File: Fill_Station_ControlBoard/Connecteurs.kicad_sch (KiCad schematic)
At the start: 44 parts, among them J1 RJ45_Wuerth_7499010211A, U1 LAN8742A, Y3 ASV-25.000MHz

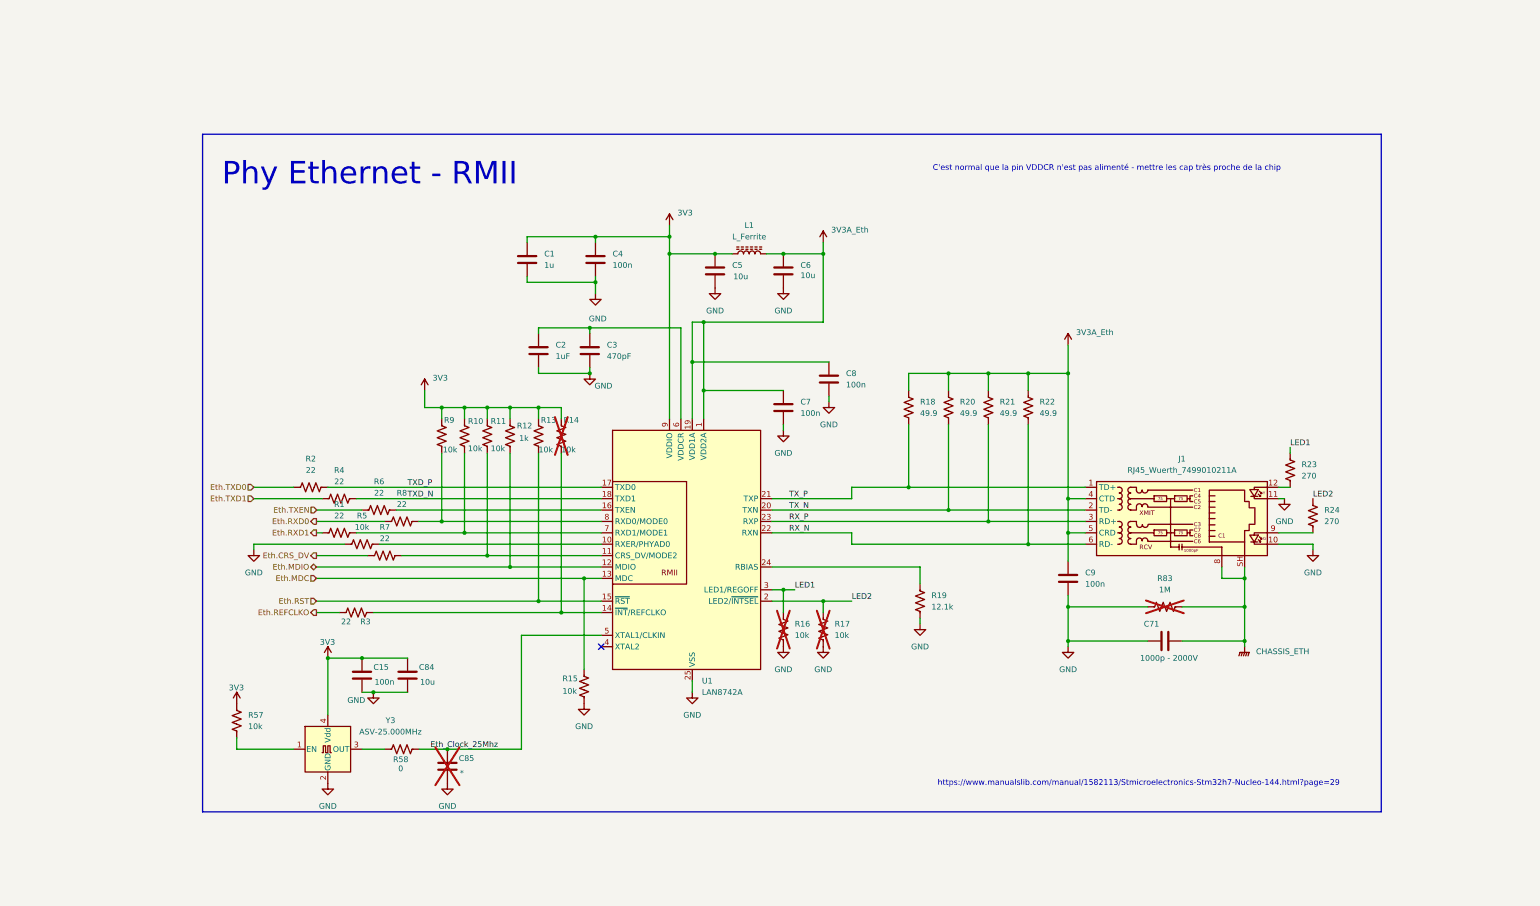
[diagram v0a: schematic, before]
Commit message: Travail Layout
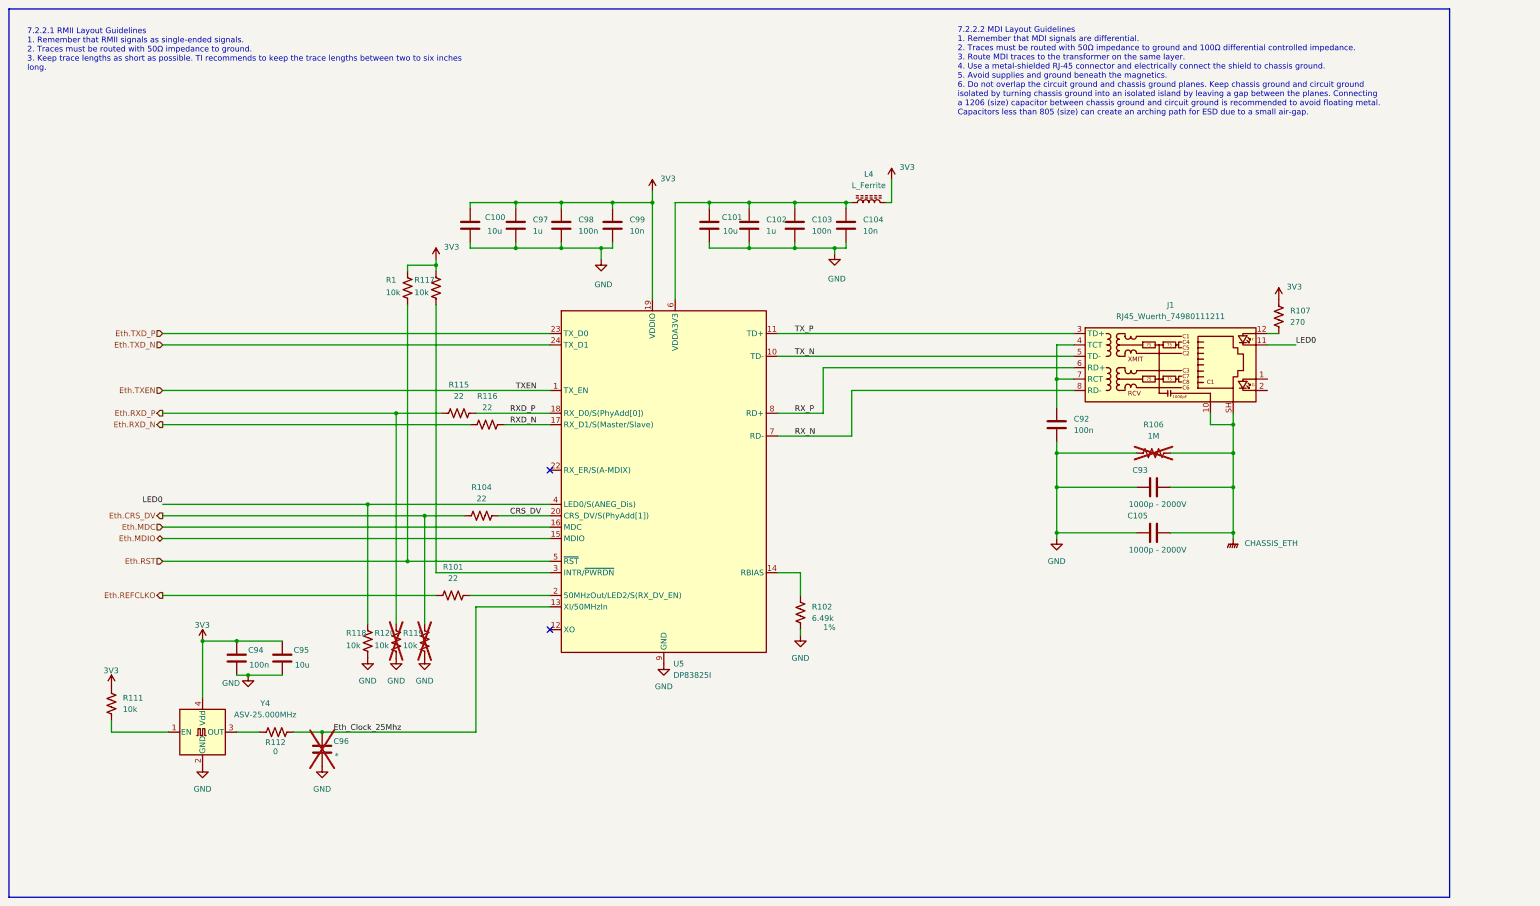
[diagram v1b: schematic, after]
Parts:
- removed C1: 1u, Capacitor_SMD:C_0603_1608Metric, symbol Device:C
- removed C15, C9: 100n, Capacitor_SMD:C_0402_1005Metric, symbol Device:C
- removed C2: 1uF, Capacitor_SMD:C_0603_1608Metric, symbol Device:C
- removed C3: 470pF, Capacitor_SMD:C_0603_1608Metric, symbol Device:C
- removed C4: 100n, Capacitor_SMD:C_0603_1608Metric, symbol Device:C
- removed C5, C6: 10u, Capacitor_SMD:C_0603_1608Metric, symbol Device:C
- removed C7, C8: 100n, Resistor_SMD:R_0402_1005Metric, symbol Device:C
- removed C71: 1000p - 2000V, Capacitor_SMD:C_1210_3225Metric, symbol Device:C
- removed C84: 10u, Capacitor_SMD:C_0402_1005Metric, symbol Device:C
- removed C85: *, Capacitor_SMD:C_0402_1005Metric, symbol Device:C
- removed J1: RJ45_Wuerth_7499010211A, Connector_RJ:RJ45_Wuerth_7499010211A_Horizontal, symbol Connector:RJ45_Wuerth_7499010211A
- removed L1: L_Ferrite, Capacitor_SMD:C_0402_1005Metric, symbol Device:L_Ferrite
- removed R10, R11, R13, R14, R15, R16, R17, R5, R9: 10k, Resistor_SMD:R_0603_1608Metric_Pad0.98x0.95mm_HandSolder, symbol Device:R_US
- removed R12: 1k, Resistor_SMD:R_0603_1608Metric_Pad0.98x0.95mm_HandSolder, symbol Device:R_US
- removed R18, R20, R21, R22: 49.9, Resistor_SMD:R_0603_1608Metric_Pad0.98x0.95mm_HandSolder, symbol Device:R_US
- removed R19: 12.1k, Resistor_SMD:R_0402_1005Metric, symbol Device:R_US
- removed R2, R3, R4, R6, R7, R8: 22, Resistor_SMD:R_0402_1005Metric, symbol Device:R_US
- removed R23, R24: 270, Resistor_SMD:R_0603_1608Metric_Pad0.98x0.95mm_HandSolder, symbol Device:R_US
- removed R57: 10k, Capacitor_SMD:C_0402_1005Metric, symbol Device:R_US
- removed R58: 0, Capacitor_SMD:C_0402_1005Metric, symbol Device:R_US
- removed R83: 1M, Resistor_SMD:R_0603_1608Metric_Pad0.98x0.95mm_HandSolder, symbol Device:R_US
- removed U1: LAN8742A, Package_DFN_QFN:VQFN-24-1EP_4x4mm_P0.5mm_EP2.5x2.5mm_ThermalVias, symbol Interface_Ethernet:LAN8742A
- removed Y3: ASV-25.000MHz, Oscillator:Oscillator_SMD_Abracon_ASV-4Pin_7.0x5.1mm, symbol Oscillator:ASV-xxxMHz
- added C100, C101: 10u, Capacitor_SMD:C_0603_1608Metric, symbol Device:C
- added C102, C97: 1u, Capacitor_SMD:C_0603_1608Metric, symbol Device:C
- added C103, C92, C94, C98: 100n, Capacitor_SMD:C_0402_1005Metric, symbol Device:C
- added C104, C99: 10n, Capacitor_SMD:C_0402_1005Metric, symbol Device:C
- added C105, C93: 1000p - 2000V, Capacitor_SMD:C_1210_3225Metric, symbol Device:C
- added C95: 10u, Capacitor_SMD:C_0402_1005Metric, symbol Device:C
- added C96: *, Capacitor_SMD:C_0402_1005Metric, symbol Device:C
- added J1: RJ45_Wuerth_74980111211, Connector_RJ:RJ45_Wuerth_74980111211_Horizontal, symbol Connector:RJ45_Wuerth_74980111211
- added L4: L_Ferrite, Capacitor_SMD:C_0402_1005Metric, symbol Device:L_Ferrite
- added R101, R104, R115, R116: 22, Resistor_SMD:R_0402_1005Metric, symbol Device:R_US
- added R102: 6.49k, Resistor_SMD:R_0402_1005Metric, symbol Device:R_US
- added R106: 1M, Resistor_SMD:R_0603_1608Metric_Pad0.98x0.95mm_HandSolder, symbol Device:R_US
- added R107: 270, Resistor_SMD:R_0603_1608Metric_Pad0.98x0.95mm_HandSolder, symbol Device:R_US
- added R111: 10k, Capacitor_SMD:C_0402_1005Metric, symbol Device:R_US
- added R112: 0, Capacitor_SMD:C_0402_1005Metric, symbol Device:R_US
- added R117, R118, R119, R120: 10k, Resistor_SMD:R_0603_1608Metric_Pad0.98x0.95mm_HandSolder, symbol Device:R_US
- added U5: DP83825I, Package_DFN_QFN:Texas_RMQ0024A_WQFN-24-1EP_3x3mm_P0.4mm_EP1.9x1.9mm, symbol Interface_Ethernet:DP83825I
- added Y4: ASV-25.000MHz, Oscillator:Oscillator_SMD_Abracon_ASV-4Pin_7.0x5.1mm, symbol Oscillator:ASV-xxxMHz
- R1: value 22 -> 10k; footprint Resistor_SMD:R_0402_1005Metric -> Resistor_SMD:R_0603_1608Metric_Pad0.98x0.95mm_HandSolder
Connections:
- net Eth.RXD1 is gone; now on net 3V3: R1.1
- net 3V3: now also C100.1, C94.1, C95.1, C97.1, C98.1, C99.1, L4.2, R107.1, R111.1, R117.1, U5.19 (VDDIO), Y4.4 (Vdd)
- net CHASSIS_ETH: now also C105.2, C93.2, J1.10, J1.SH, R106.2
- net Eth.CRS_DV: now also R104.1, R119.1
- net Eth.MDC: now also U5.16 (MDC)
- net Eth.MDIO: now also U5.15 (MDIO)
- net Eth.REFCLKO: now also R101.1
- net Eth.RST: now also R1.2, U5.5 (~{RST})
- net Eth.TXEN: now also U5.1 (TX_EN)
- net Eth_Clock_25Mhz: now also C96.1, R112.2, U5.13 (XI/50MHzIn)
- net GND: now also C100.2, C101.2, C102.2, C103.2, C104.2, C105.1, C92.2, C93.1, C94.2, C95.2, C96.2, C97.2, C98.2, C99.2, R102.2, R106.1, R118.2, R119.2, R120.2, U5.21 (GND), U5.25 (GND), U5.9 (GND), Y4.2 (GND)
- net RX_N: now also J1.8 (RD-), U5.7 (RD-)
- net RX_P: now also J1.6 (RD+), U5.8 (RD+)
- net TX_N: now also J1.5 (TD-), U5.10 (TD-)
- net TX_P: now also J1.3 (TD+), U5.11 (TD+)
- new net: C101.1, C102.1, C103.1, C104.1, L4.1, U5.6 (VDDA3V3)
- new net: R111.2, Y4.1 (EN)
- new net: R112.1, Y4.3 (OUT)
- new net: J1.12, R107.2
- new net: C92.1, J1.4 (TCT), J1.7 (RCT)
- new net: R101.2, U5.2 (50MHzOut/LED2/S(RX_DV_EN))
- new net: R102.1, U5.14 (RBIAS)
- new net: R117.2, U5.3 (INTR/~{PWRDN})
- new net CRS_DV: R104.2, U5.20 (CRS_DV/S(PhyAdd[1]))
- new net Eth.RXD_N: R116.1
- new net Eth.RXD_P: R115.1, R120.1
- new net Eth.TXD_N: U5.24 (TX_D1)
- new net Eth.TXD_P: U5.23 (TX_D0)
- new net LED0: J1.11, R118.1, U5.4 (LED0/S(ANEG_Dis))
- new net RXD_N: R116.2, U5.17 (RX_D1/S(Master/Slave))
- new net RXD_P: R115.2, U5.18 (RX_D0/S(PhyAdd[0]))
- no-connect marks 1 -> 2
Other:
- note added: "7.2.2.1 RMII Layout Guidelines 1. Remember that RMII signals as single-ended signals. 2. Traces must be routed with 50Ω impedance to ground. 3. Keep trace lengths as short as possible. TI recommends to keep the trace lengths between two to six inches long."
- note added: "7.2.2.2 MDI Layout Guidelines 1. Remember that MDI signals are differential. 2. Traces must be routed with 50Ω impedance to ground and 100Ω differential controlled impedance. 3. Route MDI traces to the transformer on the same layer. 4. Use a metal-shielded RJ-45 connector and electrically connect the shield to chassis ground. 5. Avoid supplies and ground beneath the magnetics. 6. Do not overlap t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"
- note removed: "C'est normal que la pin VDDCR n'est pas alimenté - mettre les cap très proche de la chip"
- note removed: "Phy Ethernet - RMII"
- note removed: "https://www.manualslib.com/manual/1582113/Stmicroelectronics-Stm32h7-Nucleo-144.html?page=29"
